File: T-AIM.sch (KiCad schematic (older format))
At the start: 21 parts, among them IC1 ATMEGA328PB-A

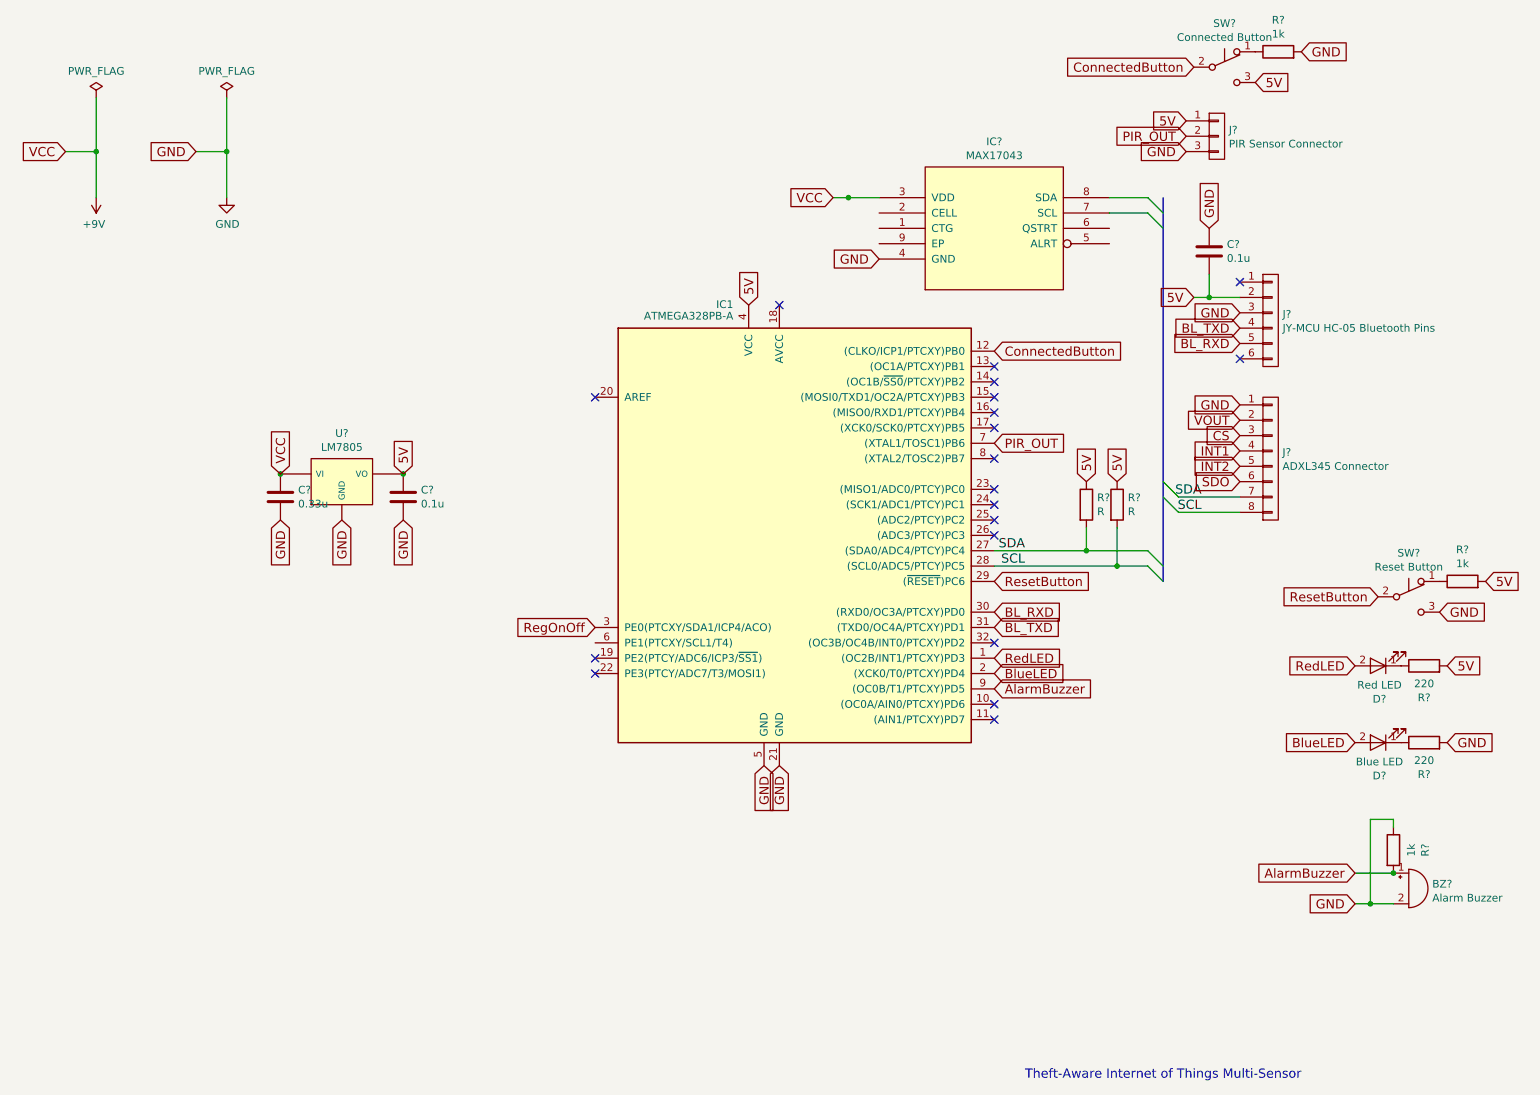
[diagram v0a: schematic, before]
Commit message: Components wired
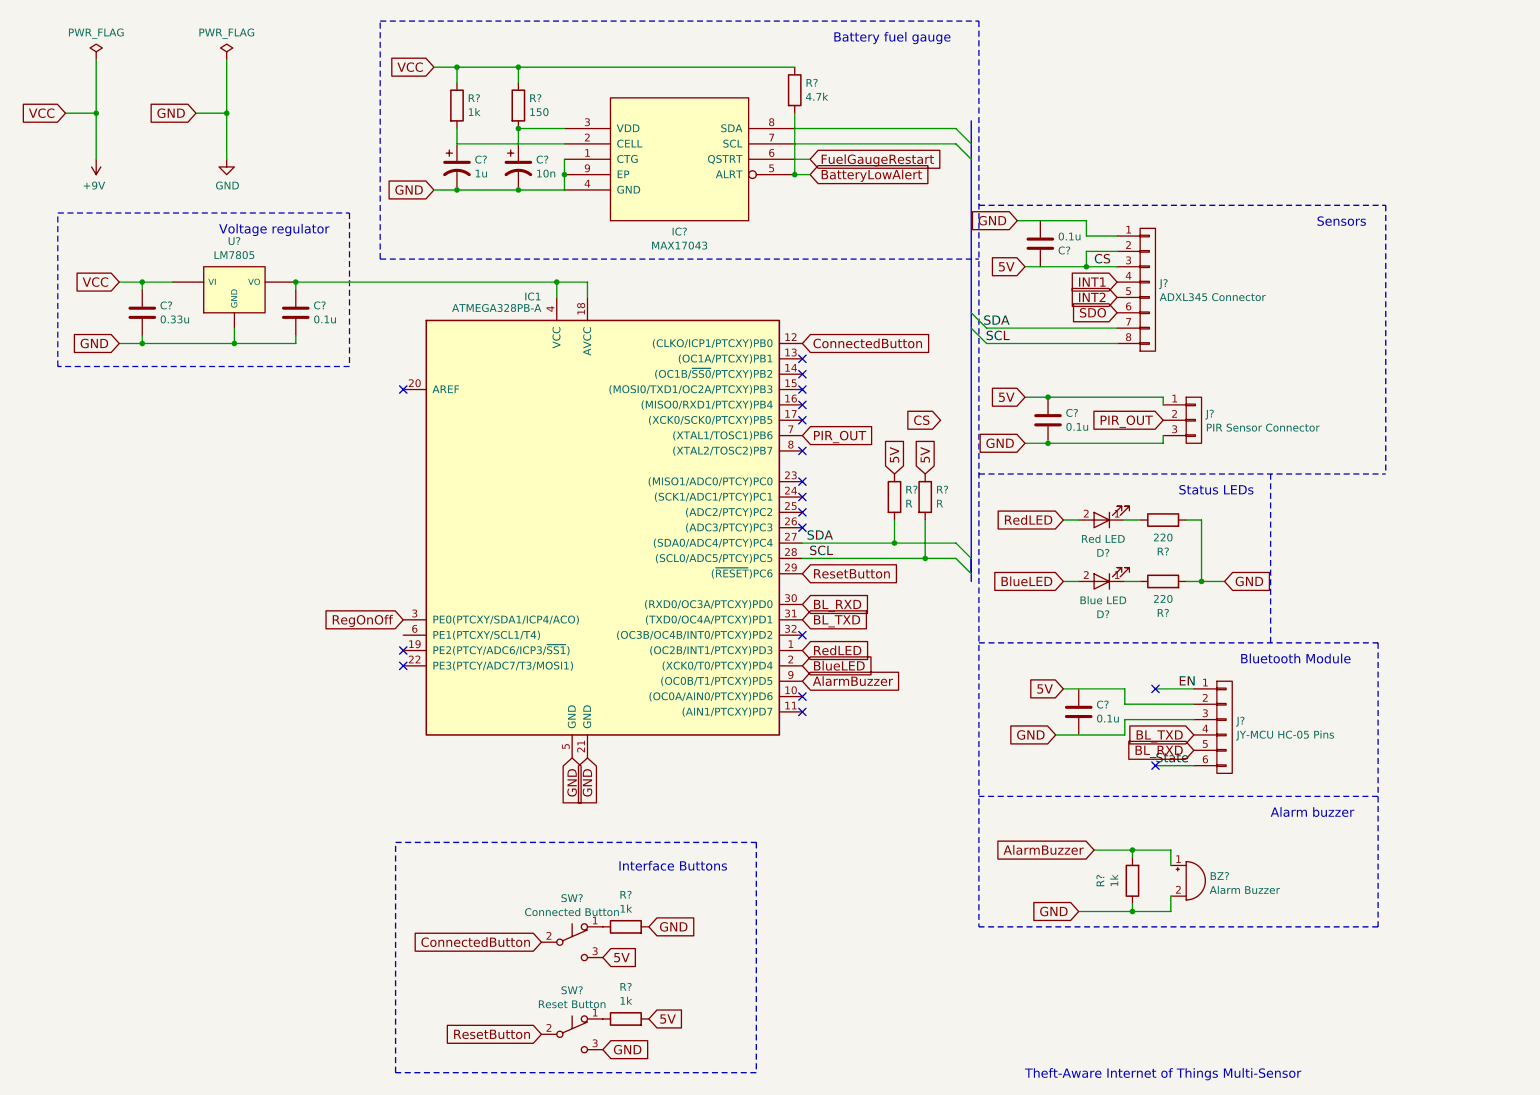
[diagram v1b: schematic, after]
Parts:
- added C?: 1u, symbol CP1
- added C?: 10n, symbol CP1
- added C? (x2): 0.1u, symbol C
- added R?: 4.7k, symbol R
- added R?: 1k, symbol R
- added R?: 150, symbol R
- J?: value JY-MCU HC-05 Bluetooth Pins -> JY-MCU HC-05 Pins
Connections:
- net CS is gone; now on net 5V: J?.3 (P3)
- net VOUT is gone; now on net 5V: J?.2 (P2)
- net +9V: now also R?.1, R?.1, R?.1; no longer IC?.3 (VDD)
- net 5V: now also C?.1; no longer C?.1, C?.2, IC1.4 (VCC), R?.2, U?.VO
- net GND: now also IC?.1 (CTG), IC?.9 (EP), R?.2, C?.2, C?.2, C?.2; no longer C?.1
- net at IC1.18 (AVCC): now also C?.1, IC1.4 (VCC), U?.VO
- net at IC?.2 (CELL): now also C?.1, R?.2
- net BatteryLowAlert: now reaches IC?.5 (ALRT)
- net BatteryLowAlert: now also R?.2
- net FuelGaugeRestart: now reaches IC?.6 (QSTRT)
- net EN: now reaches J?.1 (P1)
- net State: now reaches J?.6 (P6)
- new net: C?.1, IC?.3 (VDD), R?.2
- no-connect marks 19 -> 18
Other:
- note added: "Alarm buzzer"
- note added: "Battery fuel gauge"
- note added: "Bluetooth Module"
- note added: "Interface Buttons"
- note added: "Sensors"
- note added: "Status LEDs"
- note added: "Voltage regulator"
- moved on the sheet: BZ?, C?, D?, IC1, IC?, J?, R?, SW?, U?
